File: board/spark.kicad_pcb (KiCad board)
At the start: 4 copper layers, 257 x 109 mm, 141 parts, among them J1 SFP+, J10 Barrel_Jack, J109 Conn_01x10, J2 SFP+, J209 Conn_01x10, J3 SFP+, J309 Conn_01x10, J4 SFP+, J409 Conn_01x10, J5 SFP+, J509 Conn_01x10, J6 SFP+, J609 Conn_01x10, J7 PTH08T221W, J8 Conn_02x30_Odd_Even, P1 CONN_02X20, P2 Conn_02x20_Odd_Even, P3 CONN_02X30, P4 Conn_02x20_Odd_Even, P5 Conn_02x20_Odd_Even, P6 CONN_02X30, SW1 SW_Push, SW2 SW_DIP_x06

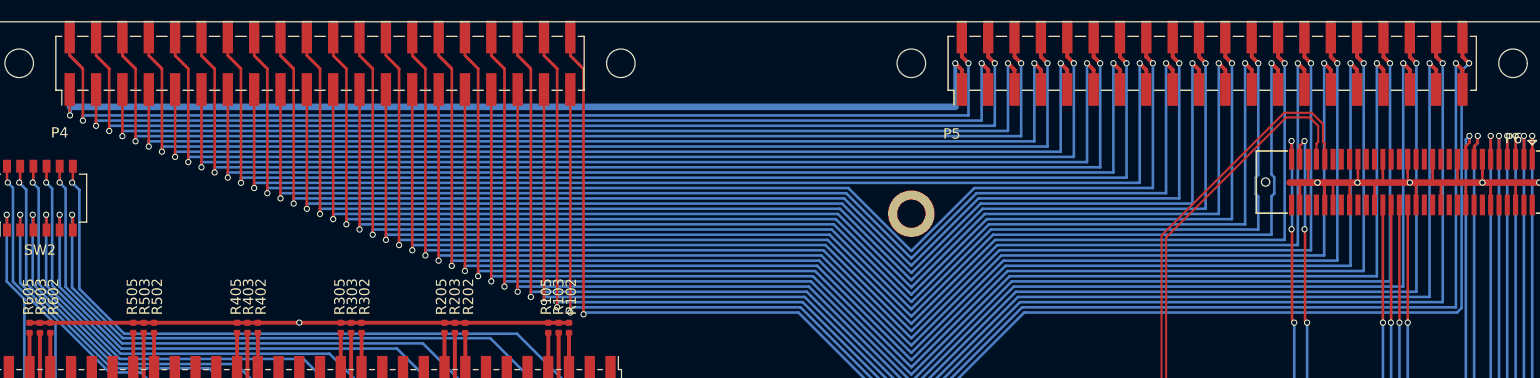
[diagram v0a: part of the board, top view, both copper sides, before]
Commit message: Release 2.0-5
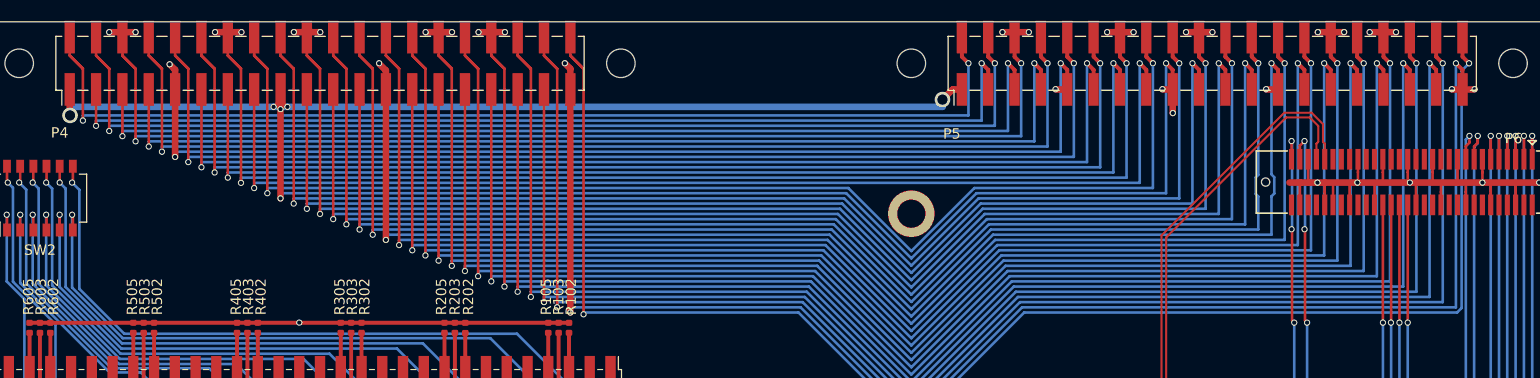
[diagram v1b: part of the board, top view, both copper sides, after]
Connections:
- P4 pad 1: Net-(P4-Pad1) -> +3V3
- P4 pad 17: Net-(P4-Pad17) -> +3V3
- P5 pad 1: Net-(P4-Pad1) -> +3V3
- P5 pad 17: Net-(P4-Pad17) -> +3V3
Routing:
- net +3V3: track 138.8 -> 354.1 mm, vias 46 -> 55
- net Net-(P4-Pad17): track 116.9 -> 0.00 mm, vias 2 -> 0
- net Net-(P4-Pad1): track 95.7 -> 0.00 mm, vias 2 -> 0
- net GND: track 1421.8 -> 1459.9 mm, vias 120 -> 147
